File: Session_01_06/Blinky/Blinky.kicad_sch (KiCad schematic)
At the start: 8 parts

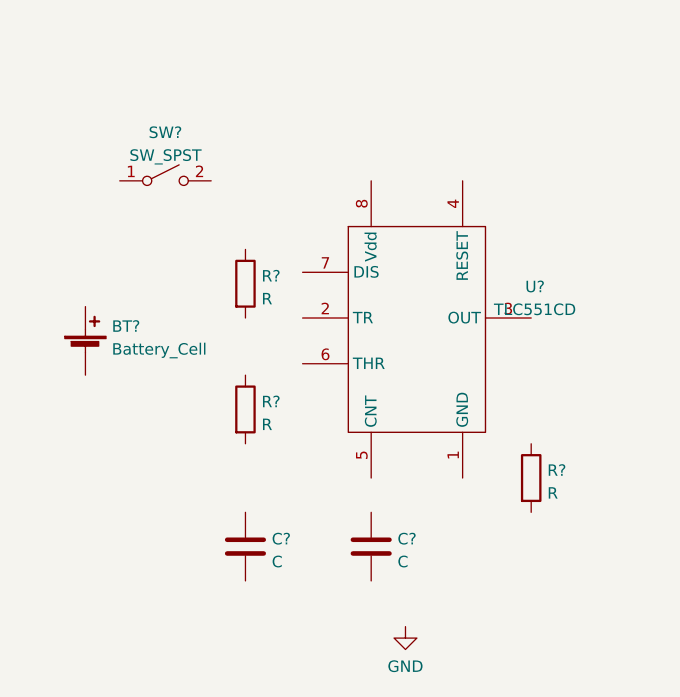
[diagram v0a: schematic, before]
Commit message: Finished the first draft of the work steps
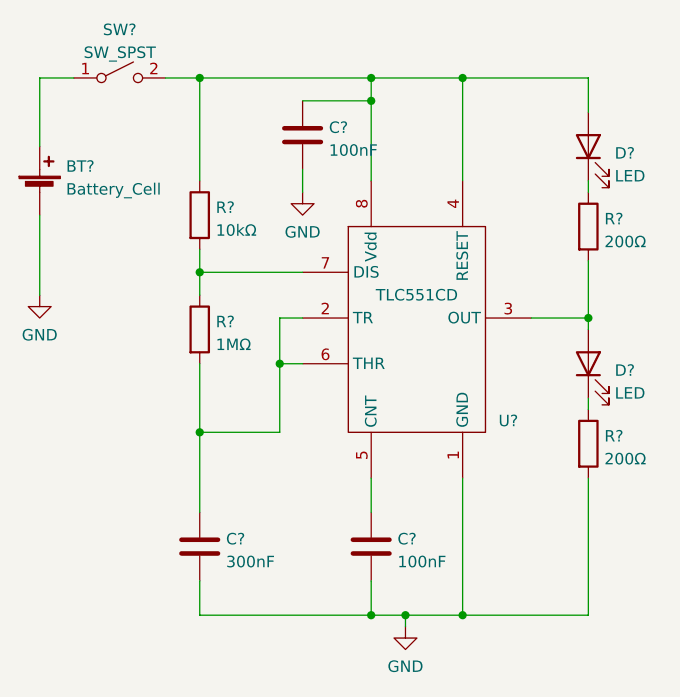
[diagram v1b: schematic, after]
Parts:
- added C?: 100nF, symbol Device:C
- added D? (x2): LED, symbol Device:LED
- added R?: 200Ω, symbol Device:R
- C?: value C -> 100nF
- C?: value C -> 300nF
- R?: value R -> 200Ω
- R?: value R -> 10kΩ
- R?: value R -> 1MΩ
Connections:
- net GND: now also BT?.2 (-), C?.2, C?.2, R?.2, U?.1 (GND), C?.2
- net at C?.1: now also U?.5 (CNT)
- net at U?.2 (TR): now also C?.1, R?.2, U?.6 (THR)
- net at U?.3 (OUT): now also D?.2 (A), R?.2
- net at U?.4 (RESET): now also R?.1, SW?.2 (B), U?.8 (Vdd), C?.1, D?.2 (A)
- net at U?.7 (DIS): now also R?.1, R?.2
- net at R?.1: now also D?.1 (K)
- net at BT?.1 (+): now also SW?.1 (A)
- new net: D?.1 (K), R?.1
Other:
- moved on the sheet: BT?, C?, R?, SW?
